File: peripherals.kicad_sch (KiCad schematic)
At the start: 36 parts, among them J5 DB25_Male_MountingHoles, J6 Conn_02x08_Odd_Even, Q25 BC856B, U16 ISL83485IBZ, U25 BSP16T1G, U29 LM358

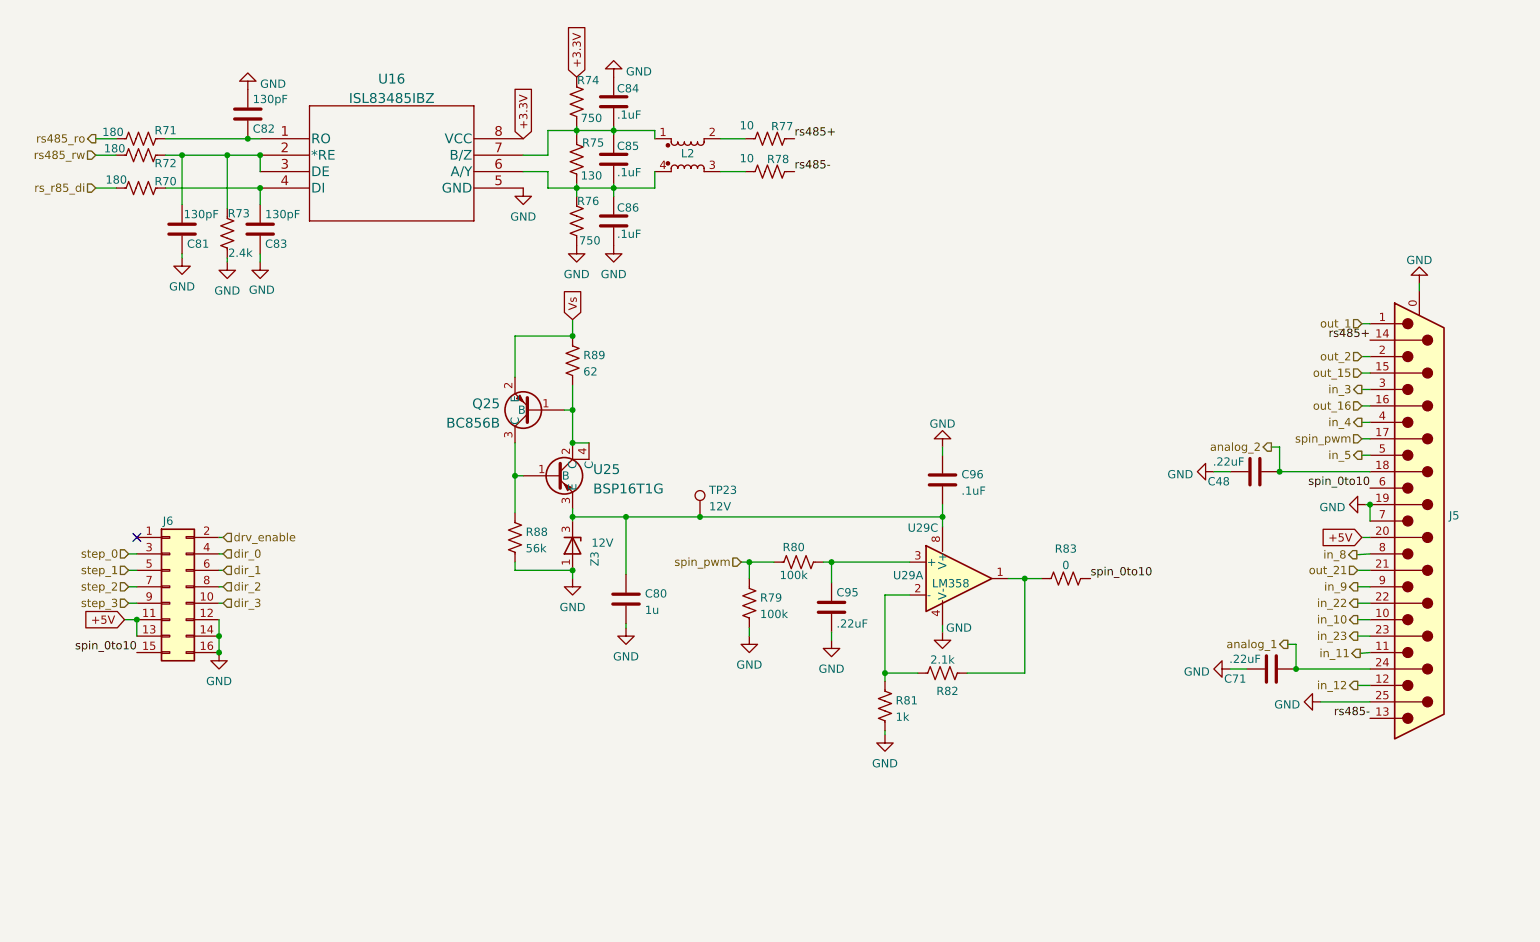
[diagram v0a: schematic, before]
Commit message: minor corrections in prep for new build
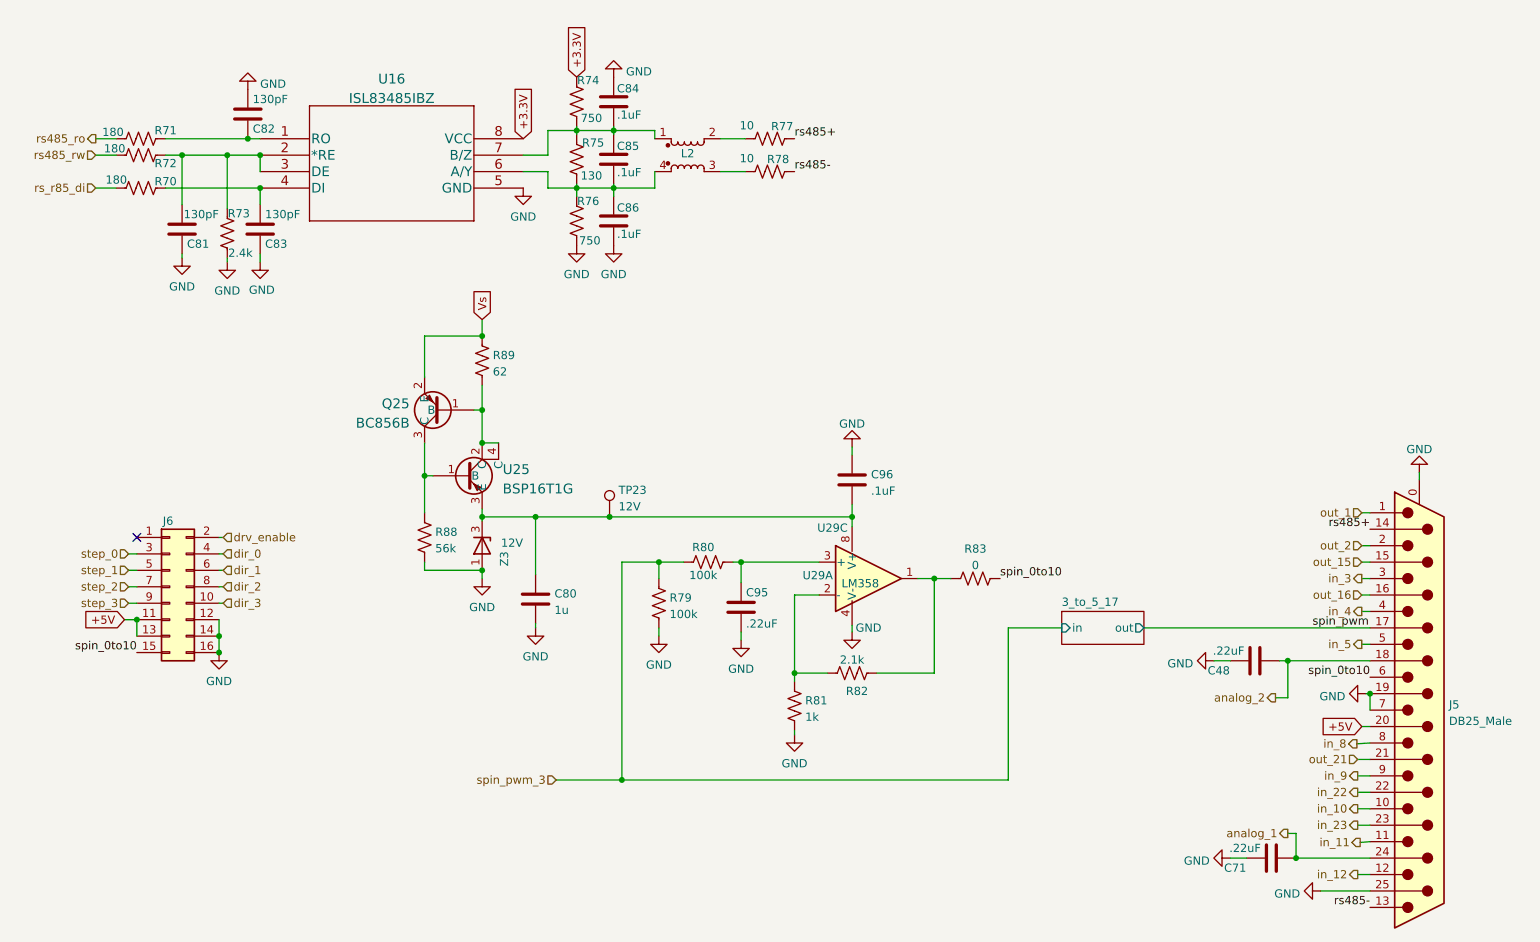
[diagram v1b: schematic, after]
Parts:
- removed J5: DB25_Male_MountingHoles, Project_Footprints_Library:182025113R161, symbol Connector:DB25_Male_MountingHoles
- added J5: DB25_Male, Project_Footprints_Library:182025113R161, symbol 1LibBBCTRL:DB25_Male
- U29: Model (none) -> LM358
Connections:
- net +5V: now also J5.20 (P20)
- net GND: now also J5.0 (PAD), J5.19 (P19), J5.25 (P25), J5.7
- net analog_1: now also J5.24 (P24)
- net analog_2: now also J5.18 (P18)
- net in_10: now also J5.10
- net in_11: now also J5.11
- net in_12: now also J5.12
- net in_22: now also J5.22 (P22)
- net in_23: now also J5.23 (P23)
- net in_3: now also J5.3
- net in_4: now also J5.4
- net in_5: now also J5.5
- net in_8: now also J5.8
- net in_9: now also J5.9
- net out_1: now also J5.1
- net out_15: now also J5.15 (P15)
- net out_16: now also J5.16 (P16)
- net out_2: now also J5.2
- net out_21: now also J5.21 (P21)
- net rs485+: now also J5.14 (P14)
- net rs485-: now also J5.13
- net spin_0to10: now also J5.6
- net spin_pwm: now also J5.17 (P17); no longer R79.2, R80.1
- new net spin_pwm_3: R79.2, R80.1
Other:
- added sheet 3_to_5_17 (level_shifter.kicad_sch)
- moved on the sheet: C48, C71, C80, C95, C96, Q25, R79, R80, R81, R82, R83, R88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

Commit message: added footprint to U29
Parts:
- C80: Model CL21B105KBFNNNE -> CC0805KKX7R7BB105
- U29: footprint (none) -> Package_SO:SOIC-8_3.9x4.9mm_P1.27mm
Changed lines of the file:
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@@
       (effects (font (size 1.27 1.27)) (justify left) hide)
     )
-    (property "Footprint" "" (id 2) (at 181.61 101.854 0)
+    (property "Footprint" "Package_SO:SOIC-8_3.9x4.9mm_P1.27mm" (id 2) (at 181.61 101.854 0)
       (effects (font (size 1.27 1.27)) hide)
     )
@@
     (property "Reference" "U29" (id 0) (at 173.7614 101.7524 0))
     (property "Value" "LM358" (id 1) (at 180.34 102.997 0))
-    (property "Footprint" "" (id 2) (at 181.61 102.235 0)
+    (property "Footprint" "Package_SO:SOIC-8_3.9x4.9mm_P1.27mm" (id 2) (at 181.61 102.235 0)
       (effects (font (size 1.27 1.27)) hide)
     )
@@
       (effects (font (size 1.27 1.27)) hide)
     )
-    (property "Datasheet" "https://media.digikey.com/pdf/Data%20Sheets/Samsung%20PDFs/CL21B105KBFNNNE_Spec.pdf" (id 3) (at 130.175 105.41 0)
-      (effects (font (size 1.27 1.27)) hide)
-    )
-    (property "Model" "CL21B105KBFNNNE" (id 4) (at 130.175 105.41 0)
-      (effects (font (size 1.27 1.27)) hide)
-    )
+    (property "Datasheet" "" (id 3) (at 130.175 105.41 0)
+      (effects (font (size 1.27 1.27)) hide)
+    )
+    (property "Model" "CC0805KKX7R7BB105" (id 4) (at 130.175 105.41 0)
+      (effects (font (size 1.27 1.27)) hide)
+    )
